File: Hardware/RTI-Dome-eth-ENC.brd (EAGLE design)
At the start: 119.4 x 71.1 mm, 77 parts, among them IC1 24AA128ST, IC3 FT232RL, IC4 REG1117, IC5 74LVC245, IC6 74ABT245, J1 POWERPOLE_POWER45A, X13 PN61729-S, X2 J1011F21PNL

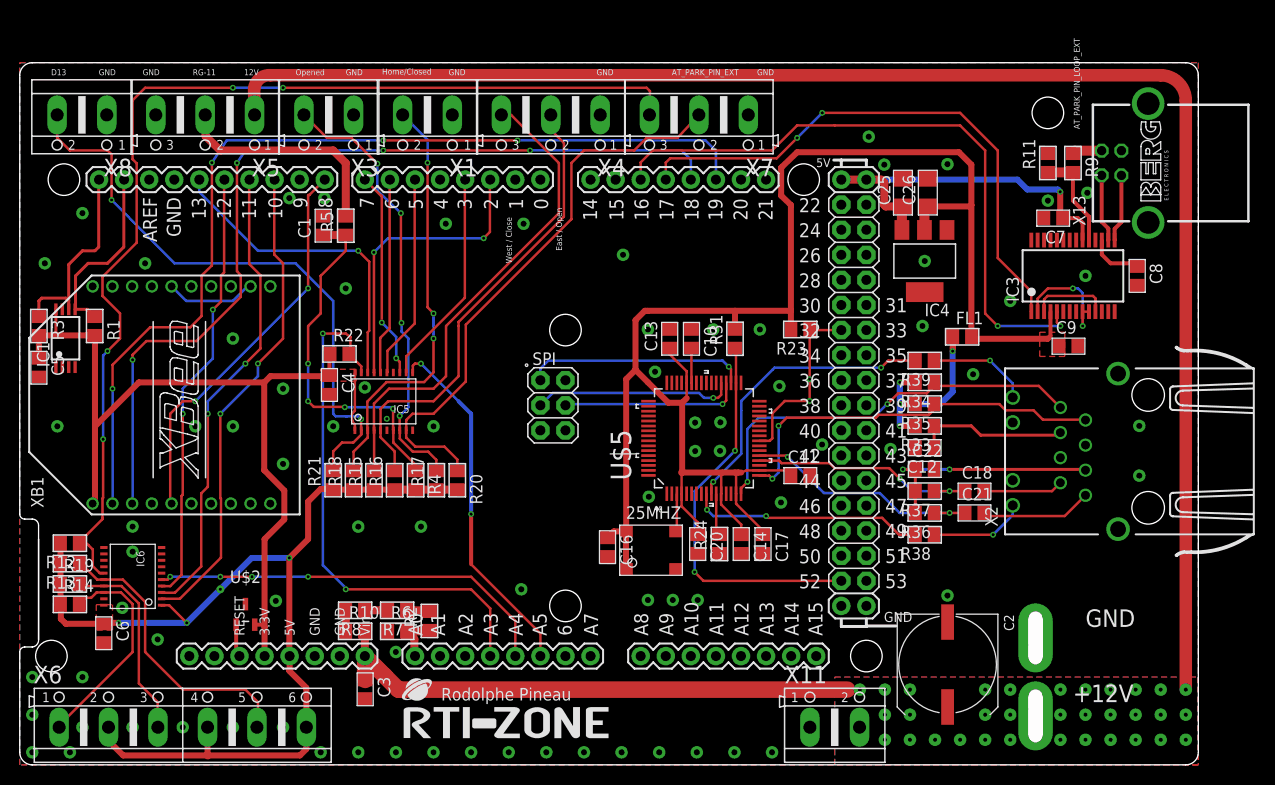
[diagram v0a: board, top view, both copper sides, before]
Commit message: Fix some componenent manufacturer reference
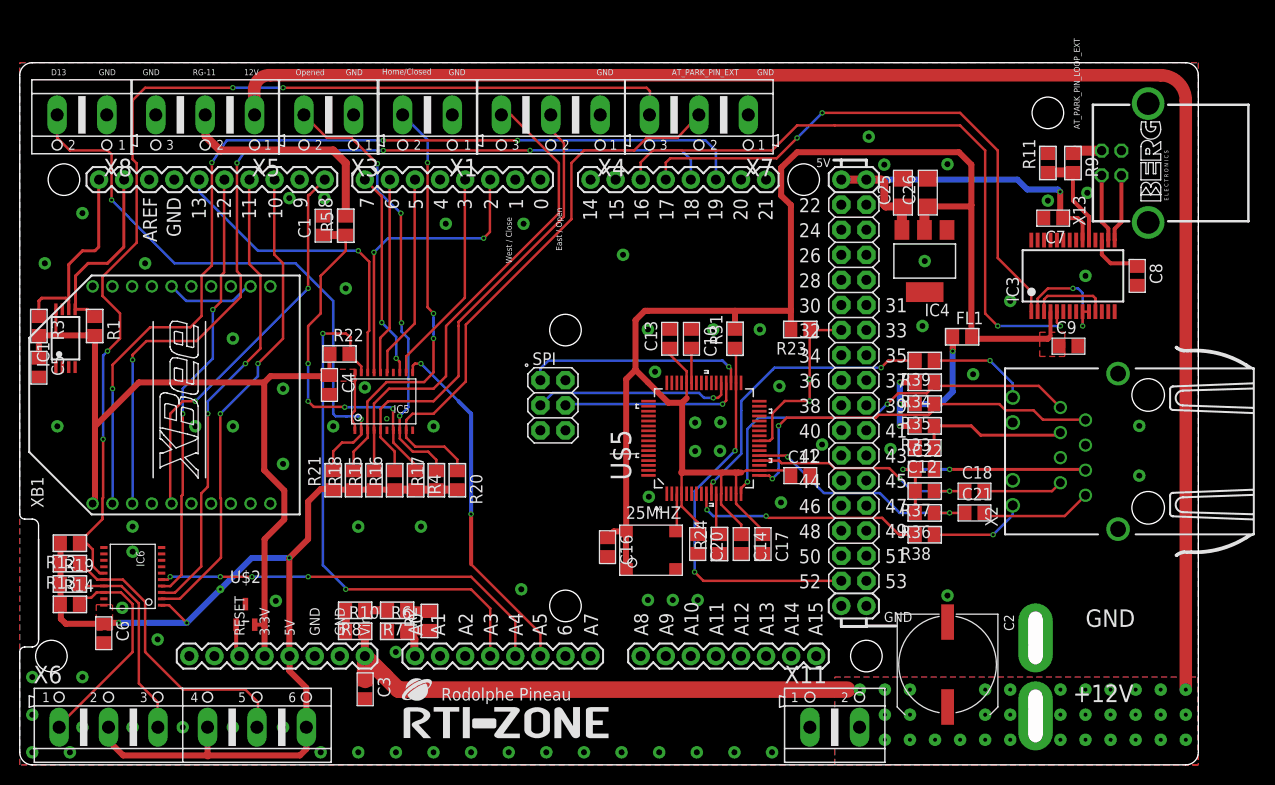
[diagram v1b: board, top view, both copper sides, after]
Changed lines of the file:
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@@
 </class>
 </classes>
-<designrules name="Fusion *">
-<description language="de">&lt;b&gt;EAGLE Design Rules&lt;/b&gt;
+<designrules name="jlcpcb2layer *">
+<description language="en">&lt;b&gt;JLCPCB Design Rules by Jaap de Dood&lt;/b&gt;
 &lt;p&gt;
-Die Standard-Design-Rules sind so gewÃÂÃÂ¤hlt, dass sie fÃÂÃÂ¼r
-die meisten Anwendungen passen. Sollte ihre Platine
-besondere Anforderungen haben, treffen Sie die erforderlichen
-Einstellungen hier und speichern die Design Rules unter
-einem neuen Namen ab.</description>
-<description language="en">&lt;b&gt;EAGLE Design Rules&lt;/b&gt;
-&lt;p&gt;
-The default Design Rules have been set to cover
-a wide range of applications. Your particular design
-may have different requirements, so please make the
-necessary adjustments and save your customized
-design rules under a new name.</description>
+Please make sure your boards conform to these design rules.
+&lt;/p&gt;</description>
 <param name="layerSetup" value="(1*16)"/>
-<param name="mtCopper" value="0.07mm 0.035mm 0.035mm 0.035mm 0.035mm 0.035mm 0.035mm 0.035mm 0.035mm 0.035mm 0.035mm 0.035mm 0.035mm 0.035mm 0.035mm 0.07mm"/>
-<param name="mtIsolate" value="1.6mm 0.5mm 0.25mm 0.15mm 0.2mm 0.15mm 0.2mm 0.15mm 0.2mm 0.15mm 0.2mm 0.15mm 0.2mm 0.25mm 0.5mm"/>
-<param name="mdWireWire" value="6mil"/>
-<param name="mdWirePad" value="6mil"/>
-<param name="mdWireVia" value="6mil"/>
-<param name="mdPadPad" value="6mil"/>
-<param name="mdPadVia" value="6mil"/>
-<param name="mdViaVia" value="6mil"/>
-<param name="mdSmdPad" value="6mil"/>
-<param name="mdSmdVia" value="6mil"/>
-<param name="mdSmdSmd" value="6mil"/>
+<param name="mtCopper" value="0.035mm 0.035mm 0.035mm 0.035mm 0.035mm 0.035mm 0.035mm 0.035mm 0.035mm 0.035mm 0.035mm 0.035mm 0.035mm 0.035mm 0.035mm 0.035mm"/>
+<param name="mtIsolate" value="1.6mm 0.15mm 0.2mm 0.15mm 0.2mm 0.15mm 0.2mm 0.15mm 0.2mm 0.15mm 0.2mm 0.15mm 0.2mm 0.15mm 0.2mm"/>
+<param name="mdWireWire" value="5mil"/>
+<param name="mdWirePad" value="5mil"/>
+<param name="mdWireVia" value="5mil"/>
+<param name="mdPadPad" value="5mil"/>
+<param name="mdPadVia" value="5mil"/>
+<param name="mdViaVia" value="5mil"/>
+<param name="mdSmdPad" value="5mil"/>
+<param name="mdSmdVia" value="5mil"/>
+<param name="mdSmdSmd" value="5mil"/>
 <param name="mdViaViaSameLayer" value="8mil"/>
 <param name="mnLayersViaInSmd" value="2"/>
-<param name="mdCopperDimension" value="13mil"/>
-<param name="mdDrill" value="6mil"/>
+<param name="mdCopperDimension" value="8mil"/>
+<param name="mdDrill" value="0.5mm"/>
 <param name="mdSmdStop" value="0mil"/>
-<param name="msWidth" value="6mil"/>
-<param name="msDrill" value="0.3mm"/>
-<param name="msMicroVia" value="8mil"/>
+<param name="msWidth" value="5mil"/>
+<param name="msDrill" value="0.2mm"/>
+<param name="msMicroVia" value="0.2mm"/>
 <param name="msBlindViaRatio" value="0.5"/>
 <param name="rvPadTop" value="0.25"/>
@@
 <param name="rvMicroViaOuter" value="0.25"/>
 <param name="rvMicroViaInner" value="0.25"/>
-<param name="rlMinPadTop" value="6mil"/>
+<param name="rlMinPadTop" value="0.13mm"/>
 <param name="rlMaxPadTop" value="20mil"/>
-<param name="rlMinPadInner" value="6mil"/>
+<param name="rlMinPadInner" value="0.13mm"/>
 <param name="rlMaxPadInner" value="20mil"/>
-<param name="rlMinPadBottom" value="6mil"/>
+<param name="rlMinPadBottom" value="0.13mm"/>
 <param name="rlMaxPadBottom" value="20mil"/>
-<param name="rlMinViaOuter" value="6mil"/>
+<param name="rlMinViaOuter" value="0.13mm"/>
 <param name="rlMaxViaOuter" value="20mil"/>
-<param name="rlMinViaInner" value="6mil"/>
+<param name="rlMinViaInner" value="0.13mm"/>
 <param name="rlMaxViaInner" value="20mil"/>
-<param name="rlMinMicroViaOuter" value="6mil"/>
+<param name="rlMinMicroViaOuter" value="0.13mm"/>
 <param name="rlMaxMicroViaOuter" value="20mil"/>
-<param name="rlMinMicroViaInner" value="6mil"/>
+<param name="rlMinMicroViaInner" value="0.13mm"/>
 <param name="rlMaxMicroViaInner" value="20mil"/>
 <param name="psTop" value="-1"/>
@@
 <param name="mvStopFrame" value="1"/>
 <param name="mvCreamFrame" value="0"/>
-<param name="mlMinStopFrame" value="0mil"/>
-<param name="mlMaxStopFrame" value="3mil"/>
-<param name="mlMinCreamFrame" value="0mil"/>
-<param name="mlMaxCreamFrame" value="3mil"/>
-<param name="mlViaStopLimit" value="130mil"/>
+<param name="mlMinStopFrame" value="0.05mm"/>
+<param name="mlMaxStopFrame" value="2.5mil"/>
+<param name="mlMinCreamFrame" value="0.05mm"/>
+<param name="mlMaxCreamFrame" value="2.5mil"/>
+<param name="mlViaStopLimit" value="40mil"/>
 <param name="srRoundness" value="0"/>
 <param name="srMinRoundness" value="0mil"/>
 <param name="srMaxRoundness" value="0mil"/>
-<param name="slThermalIsolate" value="8mil"/>
+<param name="slThermalIsolate" value="10mil"/>
 <param name="slThermalsForVias" value="0"/>
 <param name="dpMaxLengthDifference" value="10mm"/>
@@
 <param name="checkFont" value="1"/>
 <param name="checkRestrict" value="1"/>
-<param name="useDiameter" value="31"/>
+<param name="useDiameter" value="13"/>
 <param name="maxErrors" value="50"/>
 </designrules>
@@
 <attribute name="MPN" value="" x="16.51" y="3.81" size="1.778" layer="27" display="off"/>
 </element>
-<element name="IC5" library="rti" package="TSSOP20" value="74LVC245" x="36.83" y="36.83" rot="R90"/>
-<element name="IC6" library="rti" package="TSSOP20" value="74ABT245" x="11.43" y="19.05" rot="R180"/>
+<element name="IC5" library="rti" package="TSSOP20" value="74LVC245" x="36.83" y="36.83" rot="R90">
+<attribute name="MPN" value="74LVC245APW,118" x="36.83" y="36.83" size="1.778" layer="27" rot="R90" display="off"/>
+</element>
+<element name="IC6" library="rti" package="TSSOP20" value="74ABT245" x="11.43" y="19.05" rot="R180">
+<attribute name="MPN" value="SN74ABT245BDWR" x="11.43" y="19.05" size="1.778" layer="27" rot="R180" display="off"/>
+</element>
 <element name="R22" library="rti" package="R0805" value="4.7K" x="32.385" y="41.62425"/>
 <element name="U$1" library="arduino_shield" package="ARDUINO_DUE_SHIELD_FULL" value="ARDUINO_DUE_SHIELD_FULL" x="38.76675" y="35.14725"/>
@@
 <element name="C17" library="rti" package="C0805" value="100nF" x="75.285" y="22.365" rot="R270"/>
 <element name="J1" library="powerpoles" package="POWERPOLE_PAIR_45A" value="POWERPOLE_POWER45A" x="102.87" y="8.89" rot="MR90"/>
-<element name="25MHZ" library="rti" package="CB3" value="CB3LV-OSCILATOR" x="63.945" y="21.105"/>
+<element name="25MHZ" library="rti" package="CB3" value="CB3LV-OSCILATOR" x="63.945" y="21.105">
+<attribute name="MPN" value="O705025MEDH4MI" x="63.945" y="21.105" size="1.778" layer="27" display="off"/>
+</element>
 <element name="C20" library="rti" package="C0805" value="100nF" x="68.67" y="22.365" rot="R270"/>
 <element name="U$2" library="MCP120T-270I_TT" package="SOT95P237X112-3N" value="MCP120T-270I_TT" x="22.86" y="15.24">
@@
 <attribute name="HEIGHT" value="mm" x="10.16" y="25.4" size="1.778" layer="27" display="off"/>
 <attribute name="MOUSER_PRICE-STOCK" value="https://www.mouser.co.uk/ProductDetail/Microchip-Technology/MCP120T-270I-TT?qs=JaP0%252BruNJH91Pwyk6aJdSA%3D%3D" x="10.16" y="25.4" size="1.778" layer="27" display="off"/>
+<attribute name="MPN" value="MCP120T-270I/TT" x="22.86" y="15.24" size="1.778" layer="27" display="off"/>
 </element>
 <element name="C13" library="rti" package="C0805" value="10nF" x="65.835" y="43.155" rot="R90"/>
@@
 <element name="R31" library="rti" package="R0805" value="10K" x="72.45" y="43.155" rot="R90"/>
 <element name="IC4" library="burr-brown" package="SOT223" value="REG1117" x="91.665" y="51.03" rot="R180">
-<attribute name="MPN" value="REG1117" x="91.665" y="51.03" size="1.778" layer="27" rot="R180" display="off"/>
+<attribute name="MPN" value="REG1117-3.3/2K5" x="91.665" y="51.03" size="1.778" layer="27" rot="R180" display="off"/>
 <attribute name="MF" value="" x="91.665" y="51.03" size="1.778" layer="27" rot="R180" display="off"/>
 <attribute name="OC_NEWARK" value="14P6981" x="91.665" y="51.03" size="1.778" layer="27" rot="R180" display="off"/>
@@
 <element name="U$5" library="Microchip_By_element14_Batch_1" package="QFP50P1200X1200X120-44N" value="ENC424J600-I/PT" x="69.3" y="33.075" rot="R90">
 <attribute name="OC_NEWARK" value="07P9120" x="69.3" y="33.075" size="1.778" layer="27" rot="R90" display="off"/>
-<attribute name="MPN" value="enc424j600-I/pt" x="69.3" y="33.075" size="1.778" layer="27" rot="R90" display="off"/>
+<attribute name="MPN" value="ENC424J600-I/PT" x="69.3" y="33.075" size="1.778" layer="27" rot="R90" display="off"/>
 <attribute name="OC_FARNELL" value="1740226" x="69.3" y="33.075" size="1.778" layer="27" rot="R90" display="off"/>
 <attribute name="PACKAGE" value="TQFP-44" x="69.3" y="33.075" size="1.778" layer="27" rot="R90" display="off"/>
